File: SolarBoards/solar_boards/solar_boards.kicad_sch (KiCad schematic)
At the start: 14 parts, among them U8 SPV1040T

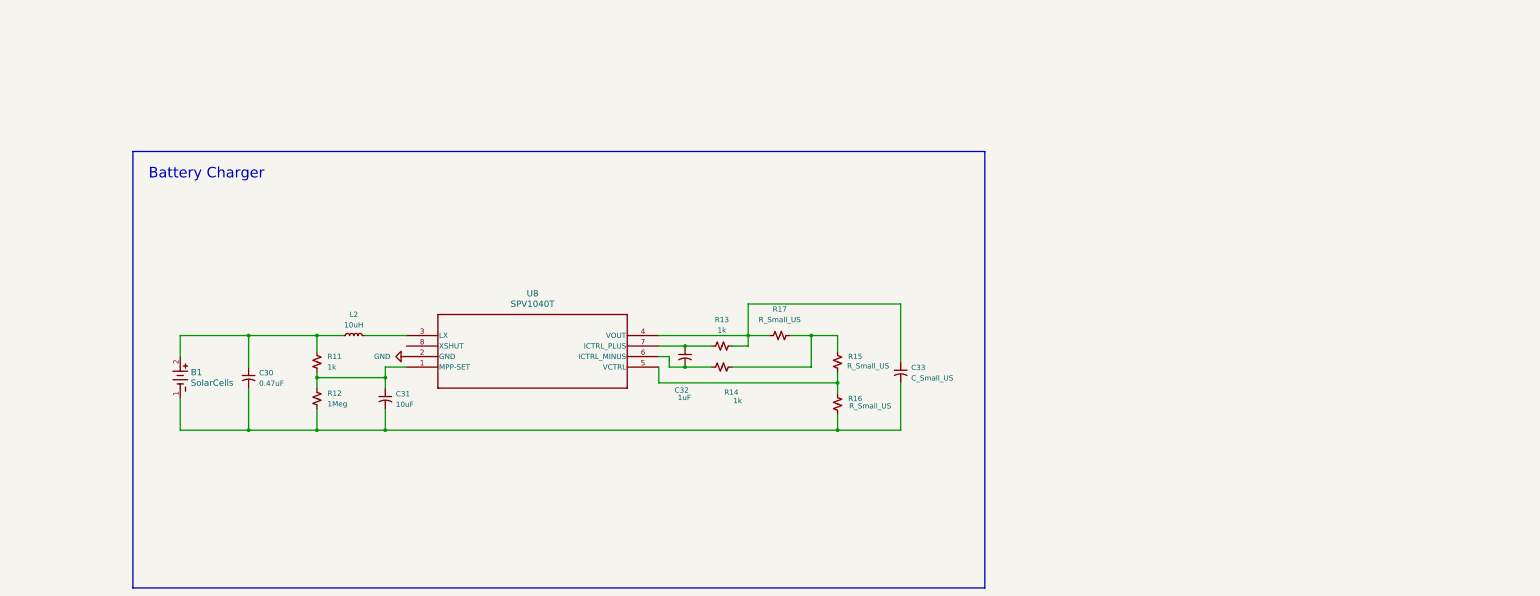
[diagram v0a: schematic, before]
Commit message: To be reviewed v0.2 to main (#3)
* Pushing Discrepancy Log

* Updated Discrepancy Log

* Update LOCK.txt

* Adjust traces to 4mil

* Adjust trace width to 4 mils

There is a courtyards overlap error with J1 and BT2. I think it will still work out

* Update LOCK.txt

* Battery Board implementation

Need to add pin assignments

* Updated thermistor footprint and added pin connections

* Changes to solar boards

* Update LOCK.txt

* started battery harvester

imported harvester and started wiring up

* began wiring

* Pushing Backplane board files

* Pushing changes to backplane

* Pushing Mainboard Split Up

Mainboard will be obsoleted soon

Battery Board and Flight Controller created

Battery Board - Good amount of routing done, additional area will be used for SuperCaps

* Modify Backplane for Battery Board

* Flight Controller updates

* Updates to FC

* some updates/ will find new solar cells

* Sorting files/ cleanup

* Updated outline

* Fixed outline

* added new boost converter and added elements

* Board sizes for FC and routing. slight Backplane changes

* boost converter values, will add solar cell

* Solar Board Schematic and Routing

* Routing and schematic work on most boards

* Finalize board work + BOM work

* STEP file additions

* Mainboard randomly got removed, added it back

---------

Co-authored-by: Christian G <tianvez273@gmail.com>
Co-authored-by: Michael Karam <michaelkaram233@gmail.com>
Co-authored-by: yoshi-here <yoshita@vt.edu>
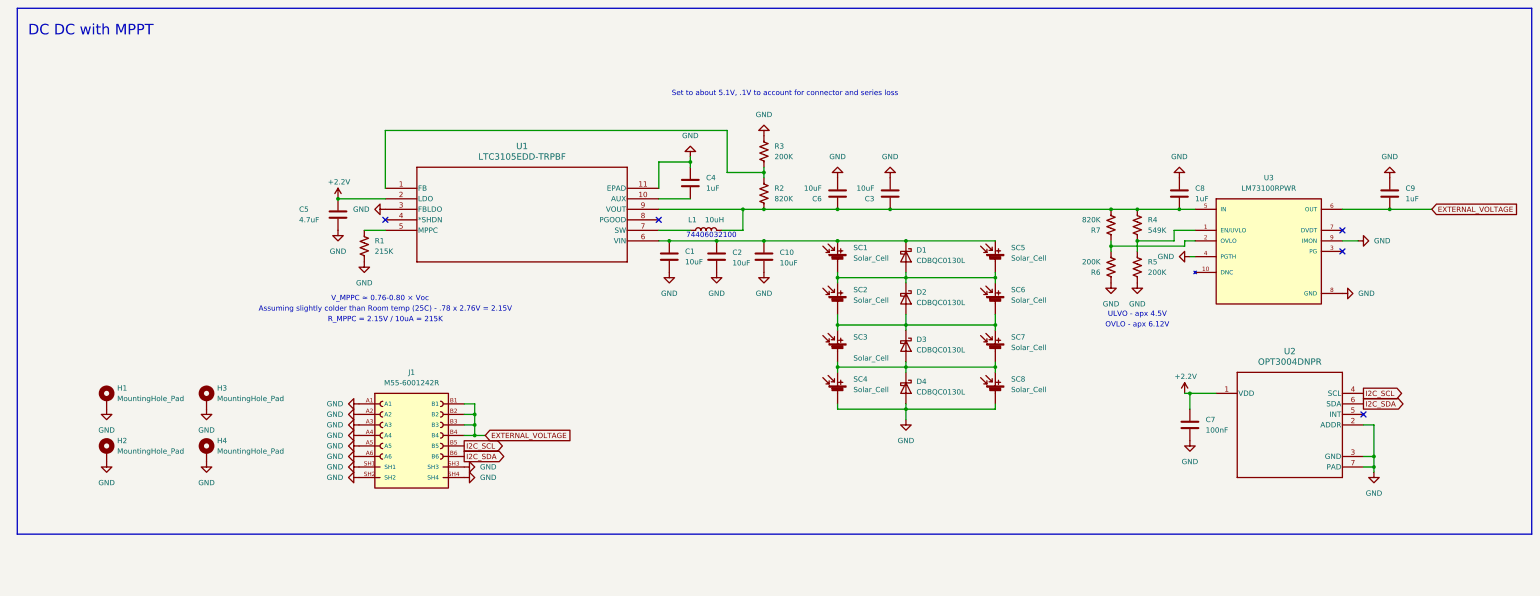
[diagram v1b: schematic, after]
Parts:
- removed B1: SolarCells, KXOB25-05X3F_IXY, symbol inspirefly:SolarCells
- removed C30: 0.47uF, symbol Device:C_Small_US
- removed C31: 10uF, symbol Device:C_Small_US
- removed C32: 1uF, symbol Device:C_Small_US
- removed C33: C_Small_US, symbol Device:C_Small_US
- removed L2: 10uH, symbol Device:L_Small
- removed R11, R13, R14: 1k, symbol Device:R_Small_US
- removed R12: 1Meg, symbol Device:R_Small_US
- removed R15, R16, R17: R_Small_US, symbol Device:R_Small_US
- removed U8: SPV1040T, SOIC_1040T_STM, symbol inspirefly:SPV1040T
- added C1, C10, C2, C3, C6: 10uF, Capacitor_SMD:C_0603_1608Metric, symbol Device:C
- added C4, C8, C9: 1uF, Capacitor_SMD:C_0402_1005Metric_Pad0.74x0.62mm_HandSolder, symbol Device:C
- added C5: 4.7uF, Capacitor_SMD:C_0603_1608Metric, symbol Device:C
- added C7: 100nF, Capacitor_SMD:C_0402_1005Metric_Pad0.74x0.62mm_HandSolder, symbol Device:C
- added D1, D2, D3, D4: CDBQC0130L, inspireFly:DIODFN100X60X55-2N, symbol Device:D_Schottky
- added H1, H2, H3, H4: MountingHole_Pad, inspireFly:MountingHole_2mm_custom, symbol Mechanical:MountingHole_Pad
- added J1: M55-6001242R, inspireFly:HARWIN_M55-6001242R, symbol inspireFly:M55-6001242R
- added L1: 10uH, inspireFly:WE-LQFS_3818, symbol Device:L
- added R1: 215K, Resistor_SMD:R_0402_1005Metric_Pad0.72x0.64mm_HandSolder, symbol Device:R_US
- added R2, R7: 820K, Resistor_SMD:R_0402_1005Metric_Pad0.72x0.64mm_HandSolder, symbol Device:R_US
- added R3, R5, R6: 200K, Resistor_SMD:R_0402_1005Metric_Pad0.72x0.64mm_HandSolder, symbol Device:R_US
- added R4: 549K, Resistor_SMD:R_0402_1005Metric_Pad0.72x0.64mm_HandSolder, symbol Device:R_US
- added SC1, SC2, SC3, SC4, SC5, SC6, SC7, SC8: Solar_Cell, inspireFly:SOLAR_KXOB25-14X1F-TR, symbol Device:Solar_Cell
- added U1: LTC3105EDD-TRPBF, inspireFly:DFN-10_DD_LIT, symbol inspireFly:LTC3105EDD-TRPBF
- added U2: OPT3004DNPR, inspireFly:DNP0006A, symbol 2026-04-11_18-01-49:OPT3004DNPR
- added U3: LM73100RPWR, inspireFly:IC_LM73100RPWR, symbol inspireFly:LM73100RPWR
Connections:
- net GND: now also C1.2, C10.2, C2.2, C3.2, C4.1, C5.2, C6.2, C7.2, C8.2, C9.2, D4.2 (A), H1.1, H2.1, H3.1, H4.1, J1.A1, J1.A2, J1.A3, J1.A4, J1.A5, J1.A6, J1.SH1, J1.SH2, J1.SH3, J1.SH4, R1.2, R3.1, R5.2, R6.1, SC4.2 (-), SC8.2 (-), U1.11 (EPAD), U1.3 (FBLDO), U2.2 (ADDR), U2.3 (GND), U2.7 (PAD), U3.4 (PGTH), U3.8 (GND), U3.9 (IMON)
- new net: C1.1, C10.1, C2.1, D1.1 (K), SC1.1 (+), SC5.1 (+), U1.6 (VIN)
- new net: D1.2 (A), D2.1 (K), SC1.2 (-), SC2.1 (+), SC5.2 (-), SC6.1 (+)
- new net: D2.2 (A), D3.1 (K), SC2.2 (-), SC3.1 (+), SC6.2 (-), SC7.1 (+)
- new net: C3.1, C6.1, C8.1, L1.2, R2.2, R4.1, R7.2, U1.9 (VOUT), U3.5 (IN)
- new net: D3.2 (A), D4.1 (K), SC3.2 (-), SC4.1 (+), SC7.2 (-), SC8.1 (+)
- new net: R2.1, R3.2, U1.1 (FB)
- new net: C4.2, U1.10 (AUX)
- new net: R1.1, U1.5 (MPPC)
- new net: L1.1, U1.7 (SW)
- new net: R4.2, R5.1, U3.1 (EN/UVLO)
- new net: R6.2, R7.1, U3.2 (OVLO)
- new net +2.2V: C5.1, C7.1, U1.2 (LDO), U2.1 (VDD)
- new net EXTERNAL_VOLTAGE: C9.1, J1.B1, J1.B2, J1.B3, J1.B4, U3.6 (OUT)
- new net I2C_SCL: J1.B5, U2.4 (SCL)
- new net I2C_SDA: J1.B6, U2.6 (SDA)
- no-connect marks 0 -> 5
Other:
- note added: "74406032100"
- note added: "Assuming slightly colder than Room temp (25C) - .78 x 2.76V = 2.15V"
- note added: "DC DC with MPPT"
- note added: "OVLO - apx 6.12V"
- note added: "R_MPPC = 2.15V / 10uA = 215K"
- note added: "Set to about 5.1V, .1V to account for connector and series loss"
- note added: "ULVO - apx 4.5V"
- note added: "V_MPPC ≈ 0.76-0.80 × Voc"
- note removed: "Battery Charger"
